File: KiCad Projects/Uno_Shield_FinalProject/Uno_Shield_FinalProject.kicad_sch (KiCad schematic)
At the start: 21 parts, among them J1 Power, J2 Digital/PWM, J3 Analog, J4 Digital/PWM, J7 MPU6050, J8 OpenLog, U1 BME280, U2 TMP36GT9

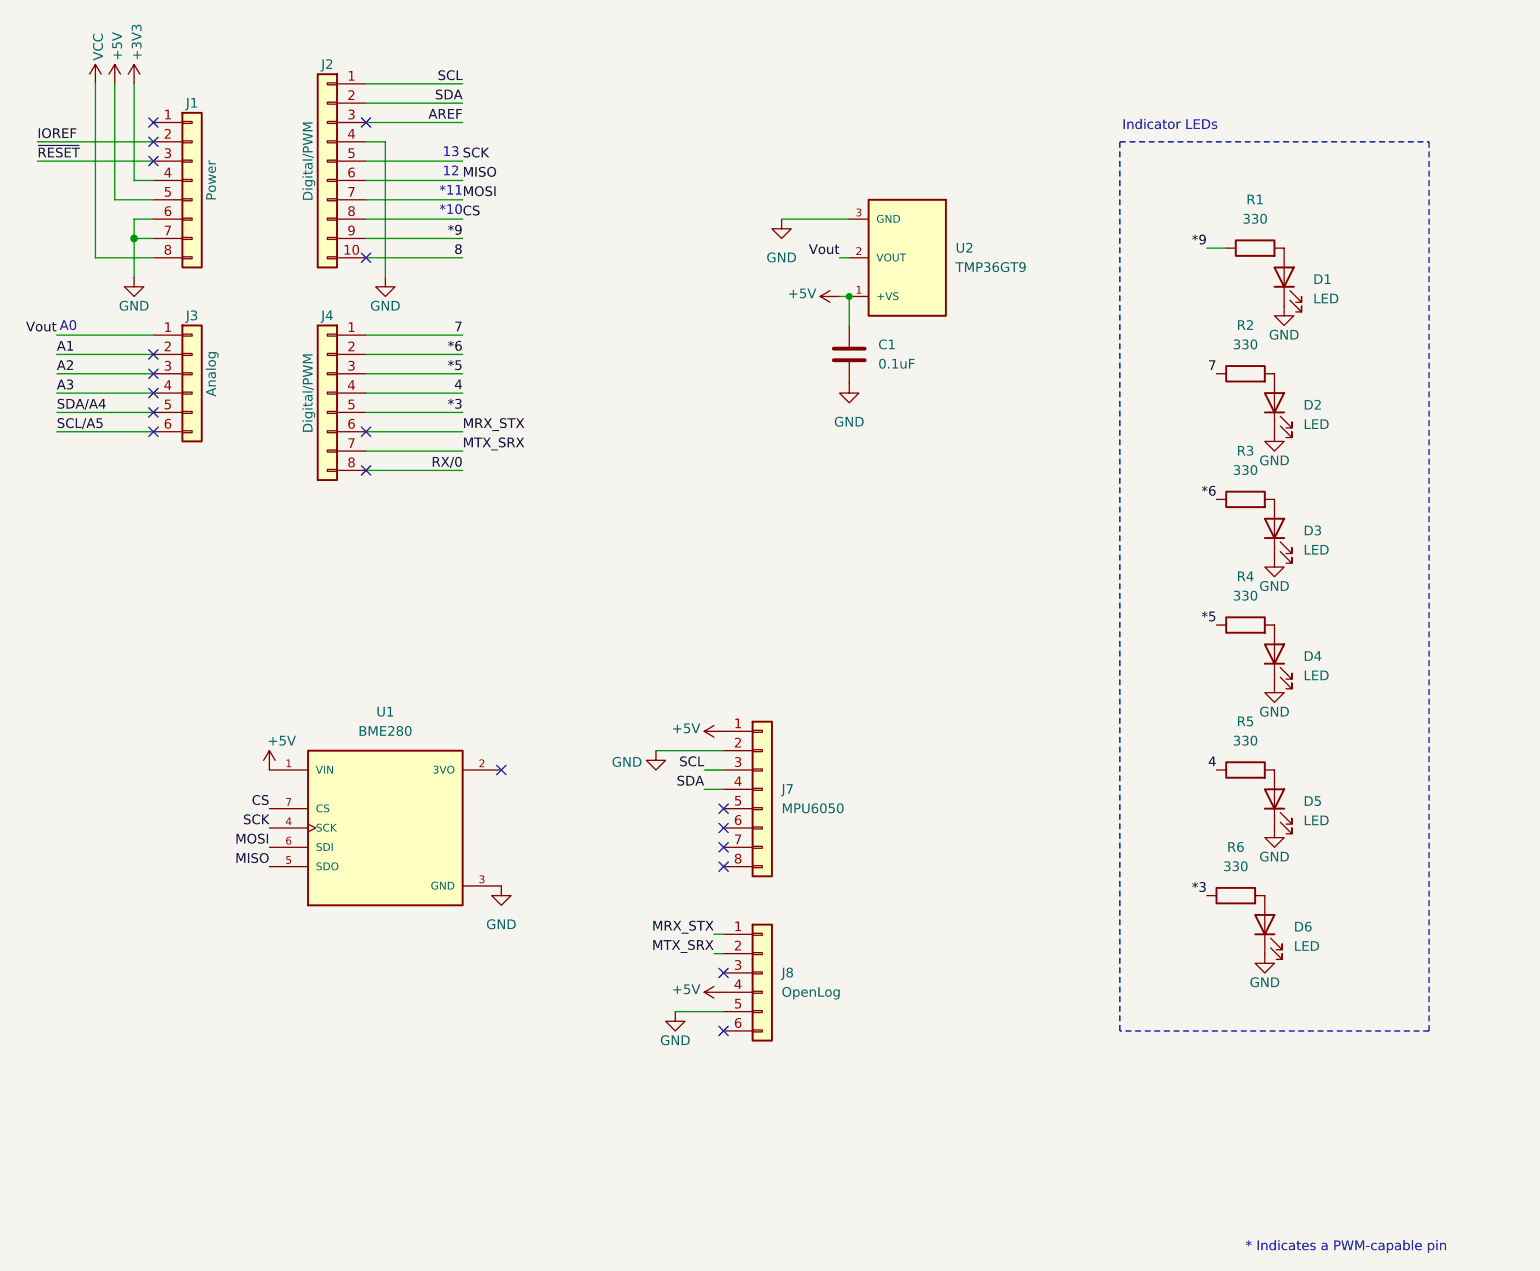
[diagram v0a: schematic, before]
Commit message: Final Project Commit
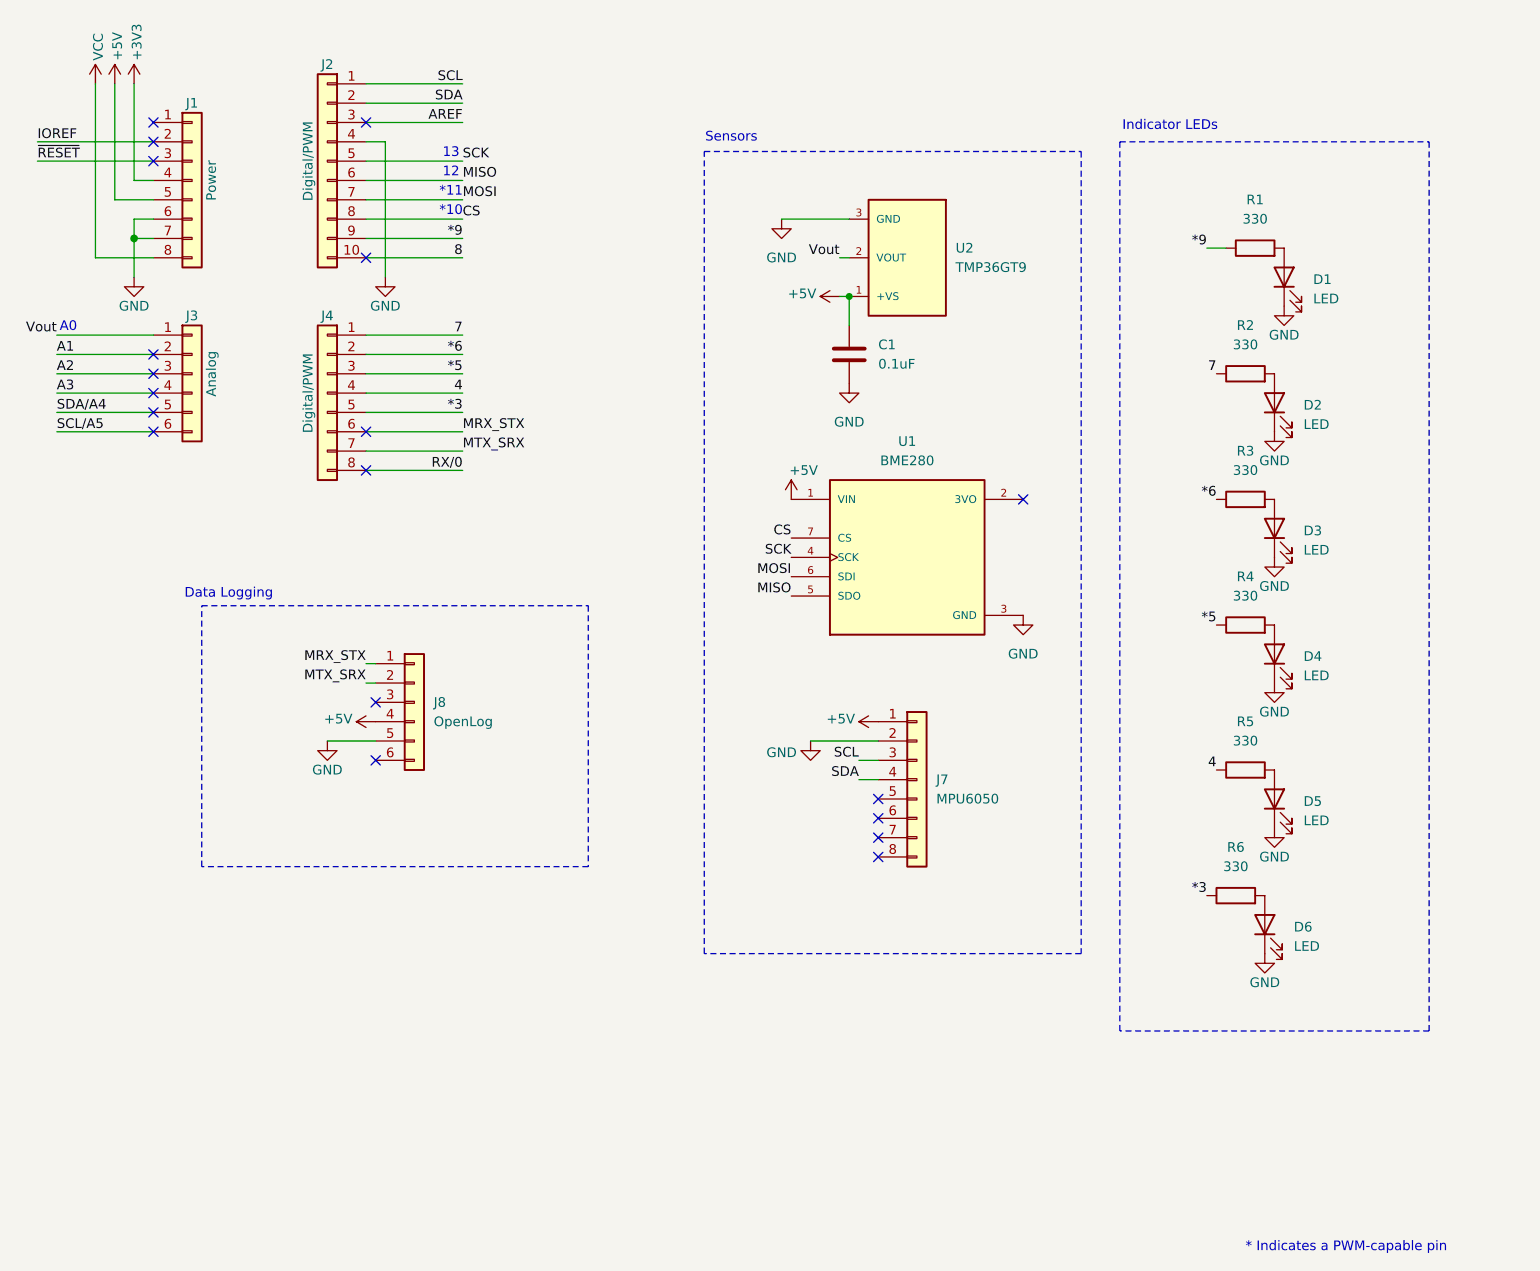
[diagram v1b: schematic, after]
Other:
- note added: "Data Logging"
- note added: "Sensors"
- moved on the sheet: J7, J8, U1
